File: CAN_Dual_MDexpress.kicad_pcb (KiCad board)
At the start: 2 copper layers, 105 x 100 mm, 134 parts, among them IC1 SI8650AB-B-IS1, IC2 A3921KLPTR-T, IC3 SI8650AB-B-IS1, IC4 A3921KLPTR-T, J1 Conn_01x02, J2 Conn_01x03, J3 Conn_01x05, J4 Conn_01x02, J5 Bus_mechaken_PCIexpress_x16_1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, Q1 NVMFD5C446NT1G, Q2 NVMFD5C446NT1G, Q3 NVMFD5C446NT1G, Q4 NVMFD5C446NT1G, U1 LDL1117S33TR_SOT223-4, U2 STM32F042K6Tx, U3 MCP2562-E-SN, U4 LDL1117S33TR_SOT223-4

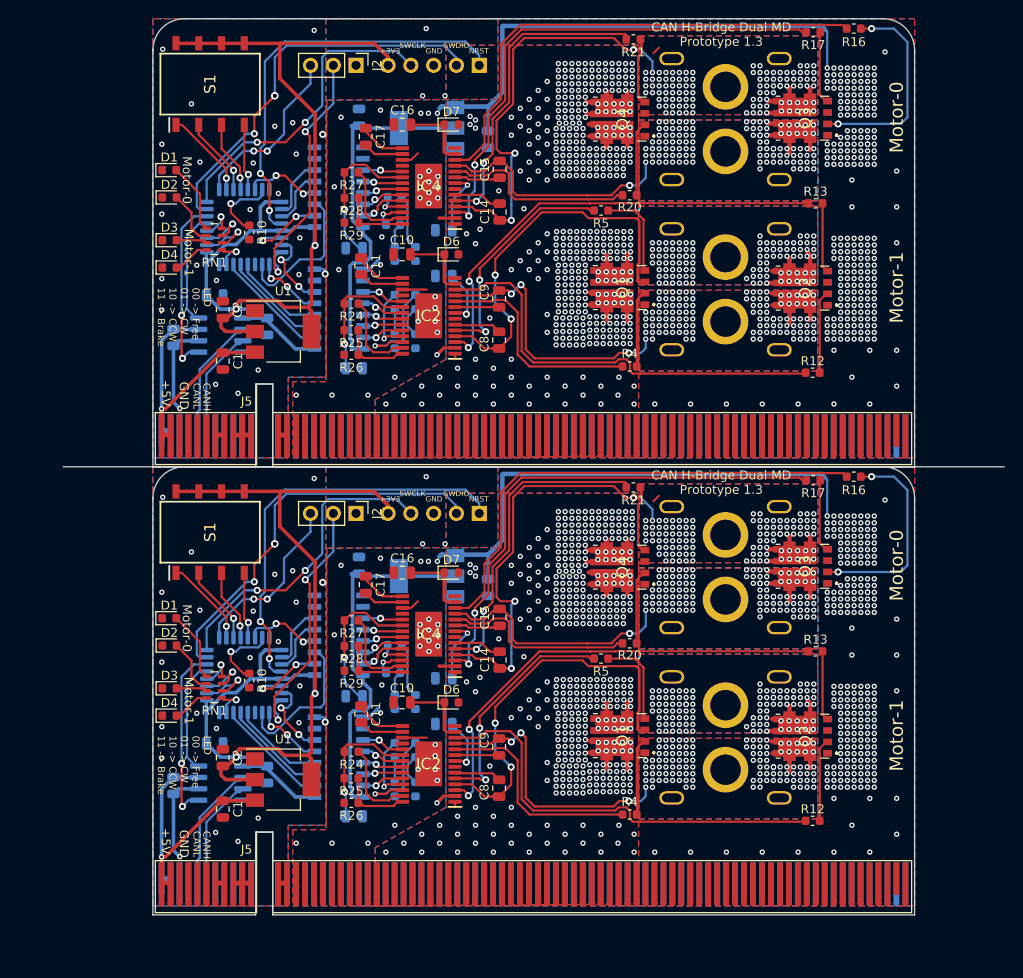
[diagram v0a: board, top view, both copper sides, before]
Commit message: Prototype 1.3
FusionPCB(12/12)
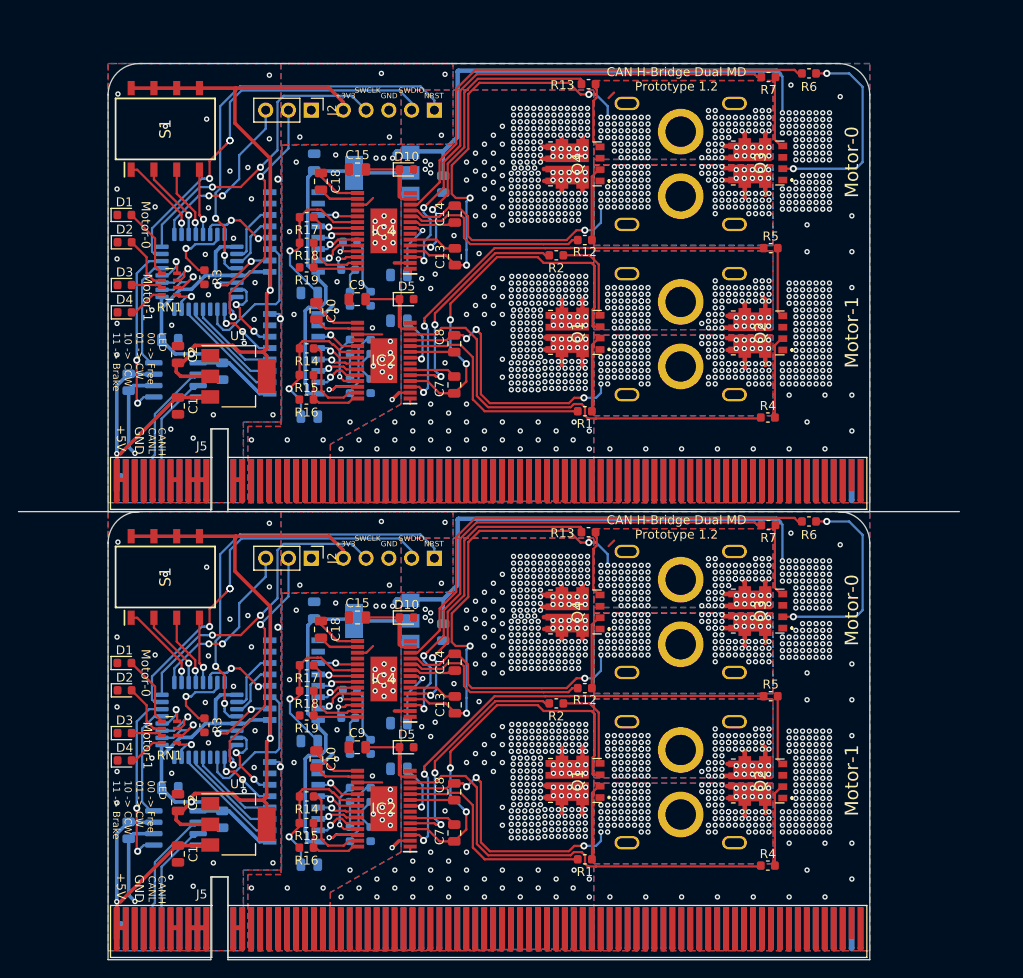
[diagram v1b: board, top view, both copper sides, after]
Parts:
- removed D11: LED, LED_SMD:LED_0603_1608Metric
- removed R20, R21: 21, Resistor_SMD:R_0603_1608Metric
- removed R24, R27: 3K, Resistor_SMD:R_0603_1608Metric
- removed R25, R28: 3.74k, Resistor_SMD:R_0603_1608Metric
- removed R26, R29: 1.2k, Resistor_SMD:R_0603_1608Metric
- removed R30, R31, R32, R33: 10K, Resistor_SMD:R_0603_1608Metric
- added D5: D, Diode_SMD:D_0603_1608Metric, F.Cu at (148.3, 66.3)
- added R1: 21, Resistor_SMD:R_0603_1608Metric, F.Cu at (168.2, 78.8)
- added R11: 10K, Resistor_SMD:R_0603_1608Metric, B.Cu at (141.8, 63.0)
- added R14: 3K, Resistor_SMD:R_0603_1608Metric, F.Cu at (137.2, 71.8)
- added R15: 3.74k, Resistor_SMD:R_0603_1608Metric, F.Cu at (137.1, 74.8)
- added R18: 3.74k, Resistor_SMD:R_0603_1608Metric, F.Cu at (137.2, 60.0)
- added R19: 1.2k, Resistor_SMD:R_0603_1608Metric, F.Cu at (137.2, 62.8)
- added R2: 21, Resistor_SMD:R_0603_1608Metric, F.Cu at (165.0, 61.4)
- added R3: 10K, Resistor_SMD:R_0603_1608Metric, F.Cu at (125.8, 63.9)
- added R6: 21, Resistor_SMD:R_0603_1608Metric, F.Cu at (193.2, 41.1)
- added R7: 21, Resistor_SMD:R_0603_1608Metric, F.Cu at (188.7, 41.5)
- added R8: 10K, Resistor_SMD:R_0603_1608Metric, B.Cu at (142.0, 71.6)
- added R9: 10K, Resistor_SMD:R_0603_1608Metric, B.Cu at (144.3, 71.6)
- C10: value 0.1uF -> 0.47uF
- C11: value 0.47uF -> 0.1uF; moved to B.Cu
- C12, C6: value 0.1uF -> 4.7uF
- C13, C7: value 4.7uF -> 0.1uF; moved to F.Cu
- C16: value 0.1uF -> 1uF; moved to B.Cu
- C17: value 0.47uF -> 4.7uF; moved to B.Cu
- C18: value 0.1uF -> 0.47uF; moved to F.Cu
- C19: value 4.7uF -> 0.1uF
- C3: value 1uF -> 0.1uF
- D10: value LED -> D; footprint LED_SMD:LED_0603_1608Metric -> Diode_SMD:D_0603_1608Metric; moved to F.Cu
- D6, D7: value D -> LED; footprint Diode_SMD:D_0603_1608Metric -> LED_SMD:LED_0603_1608Metric; moved to B.Cu
- R10: moved to B.Cu
- R16: value 21 -> 1.2k
- R17: value 21 -> 3K
- moved R16 73.8 mm to (137.1, 77.5), turned to 180 degrees
- moved R17 60.2 mm to (137.2, 57.1)
- moved C3 42.0 mm to (121.9, 70.9), turned to 180 degrees
- moved D7 30.5 mm to (144.3, 76.0), turned to 90 degrees
- moved R12 29.4 mm to (168.2, 59.7)
- moved R13 28.6 mm to (168.6, 42.3)
- moved C6 25.2 mm to (147.5, 68.7), turned to 180 degrees
- moved C19 20.4 mm to (137.5, 65.6), turned to 180 degrees
- moved R5 19.4 mm to (188.9, 60.6)
- moved D10 19.2 mm to (148.3, 51.8), turned to 0 degrees
- moved D6 18.5 mm to (142.0, 76.0), turned to 90 degrees
- moved C11 17.8 mm to (137.5, 79.4), turned to 0 degrees
- moved C5 16.6 mm to (117.3, 75.6)
- moved R4 16.4 mm to (188.6, 79.5)
- moved C15 15.9 mm to (142.8, 51.8), turned to 180 degrees
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- renumbered C11 to C10, C12 to C11, C13 to C12, C14 to C13, C15 to C14, C16 to C15, C3 to C16, C19 to C17, C17 to C18, C18 to C19, C4 to C3, C5 to C4, C6 to C5, C7 to C6, C8 to C7, C9 to C8, C10 to C9, D7 to D10, D6 to D5, D10 to D6, D11 to D7, R4 to R1, R30 to R10, R31 to R11, R20 to R12, R21 to R13, R24 to R14, R25 to R15, R26 to R16, R27 to R17, R28 to R18, R29 to R19, R5 to R2, R10 to R3, R12 to R4, R13 to R5, R16 to R6, R17 to R7, R32 to R8, R33 to R9
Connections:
- C10 pad 2: GNDPWR -> Net-(C10-Pad2)
- C10 pad 1: Net-(C11-Pad1) -> Net-(C10-Pad1)
- C10 pad 2: Net-(C11-Pad2) -> Net-(C10-Pad2)
- C11 pad 2: Net-(C11-Pad2) -> GNDPWR
- C11 pad 1: Net-(C12-Pad1) -> Net-(C11-Pad1)
- C12 pad 1: Net-(C12-Pad1) -> VREG_0
- C13 pad 1: VREG_0 -> SB_0
- C13 pad 2: GNDPWR -> Net-(C13-Pad2)
- C13 pad 2: Net-(C14-Pad2) -> Net-(C13-Pad2)
- C14 pad 1: SB_0 -> Net-(C14-Pad1)
- C14 pad 2: Net-(C14-Pad2) -> SA_0
- C14 pad 1: Net-(C15-Pad1) -> Net-(C14-Pad1)
- C15 pad 2: SA_0 -> GNDPWR
- C15 pad 1: Net-(C16-Pad1) -> Net-(C15-Pad1)
- C16 pad 1: Net-(C16-Pad1) -> VCC
- C17 pad 1: Net-(C17-Pad1) -> GNDPWR
- C17 pad 2: Net-(C17-Pad2) -> MD_3V3
- C18 pad 2: GNDPWR -> Net-(C18-Pad2)
- C18 pad 1: Net-(C17-Pad1) -> Net-(C18-Pad1)
- C18 pad 2: Net-(C17-Pad2) -> Net-(C18-Pad2)
- C19 pad 1: GNDPWR -> Net-(C19-Pad1)
- C19 pad 2: MD_3V3 -> GNDPWR
- C19 pad 1: Net-(C18-Pad1) -> Net-(C19-Pad1)
- C3 pad 1: VCC -> GND
- C3 pad 2: GNDPWR -> +3V3
- C5 pad 2: +3V3 -> +5V
- C6 pad 1: GND -> VREG_1
- C6 pad 2: +5V -> GNDPWR
- C7 pad 1: VREG_1 -> SB_1
- C7 pad 2: GNDPWR -> Net-(C7-Pad2)
- C7 pad 2: Net-(C8-Pad2) -> Net-(C7-Pad2)
- C8 pad 1: SB_1 -> SA_1
- C8 pad 2: Net-(C9-Pad2) -> Net-(C8-Pad2)
- C9 pad 1: SA_1 -> Net-(C9-Pad1)
- C9 pad 2: Net-(C9-Pad2) -> GNDPWR
- C9 pad 1: Net-(C10-Pad1) -> Net-(C9-Pad1)
- D10 pad 1: GNDPWR -> Net-(C15-Pad1)
- D10 pad 2: Net-(D10-Pad2) -> VCC
- D10 pad 1: Net-(C16-Pad1) -> Net-(C15-Pad1)
- D5 pad 1: Net-(C10-Pad1) -> Net-(C9-Pad1)
- D6 pad 1: Net-(C10-Pad1) -> GNDPWR
- D6 pad 2: VCC -> Net-(D6-Pad2)
- D6 pad 2: Net-(D10-Pad2) -> Net-(D6-Pad2)
- D7 pad 1: Net-(C16-Pad1) -> GNDPWR
- D7 pad 2: VCC -> Net-(D7-Pad2)
- D7 pad 2: Net-(D11-Pad2) -> Net-(D7-Pad2)
- IC2 pad 13: Net-(C10-Pad1) -> Net-(C9-Pad1) (x2)
- IC2 pad 15: Net-(C11-Pad1) -> Net-(C10-Pad1) (x2)
- IC2 pad 16: Net-(C11-Pad2) -> Net-(C10-Pad2) (x2)
- IC2 pad 20: Net-(C12-Pad1) -> Net-(C11-Pad1) (x2)
- IC2 pad 6: Net-(C8-Pad2) -> Net-(C7-Pad2) (x2)
- IC2 pad 9: Net-(C9-Pad2) -> Net-(C8-Pad2) (x2)
- IC4 pad 13: Net-(C16-Pad1) -> Net-(C15-Pad1) (x2)
- IC4 pad 15: Net-(C17-Pad1) -> Net-(C18-Pad1) (x2)
- IC4 pad 16: Net-(C17-Pad2) -> Net-(C18-Pad2) (x2)
- IC4 pad 20: Net-(C18-Pad1) -> Net-(C19-Pad1) (x2)
- IC4 pad 6: Net-(C14-Pad2) -> Net-(C13-Pad2) (x2)
- IC4 pad 9: Net-(C15-Pad1) -> Net-(C14-Pad1) (x2)
- R10 pad 1: /BOOT -> MD_FF1_0
- R10 pad 2: GND -> Net-(D8-Pad2)
- R12 pad 1: GLA_1 -> GHA_0
- R12 pad 2: Net-(Q2-Pad2) -> Net-(Q4-Pad2)
- R13 pad 1: Net-(Q2-Pad4) -> Net-(Q4-Pad4)
- R13 pad 2: GLB_1 -> GHB_0
- R14 pad 2: Net-(C12-Pad1) -> Net-(C11-Pad1)
- R15 pad 2: Net-(C12-Pad1) -> Net-(C11-Pad1)
- R16 pad 1: GLA_0 -> Net-(IC2-Pad28)
- R16 pad 2: Net-(Q3-Pad2) -> GNDPWR
- R17 pad 1: Net-(Q3-Pad4) -> Net-(IC4-Pad27)
- R17 pad 2: GLB_0 -> Net-(C19-Pad1)
- R17 pad 2: Net-(C18-Pad1) -> Net-(C19-Pad1)
- R18 pad 2: Net-(C18-Pad1) -> Net-(C19-Pad1)
- R4 pad 1: GHA_1 -> GLA_1
- R4 pad 2: Net-(Q1-Pad2) -> Net-(Q2-Pad2)
- R5 pad 1: Net-(Q1-Pad4) -> Net-(Q2-Pad4)
- R5 pad 2: GHB_1 -> GLB_1
- R8 pad 2: Net-(D10-Pad2) -> Net-(D6-Pad2)
- R9 pad 2: Net-(D11-Pad2) -> Net-(D7-Pad2)
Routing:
- net Net-(C19-Pad1): track 0.00 -> 36.0 mm, vias 0 -> 2
- net Net-(C12-Pad1): track 29.2 -> 0.00 mm, vias 2 -> 0
- net Net-(C18-Pad1): track 33.8 -> 11.0 mm, vias 2 -> 0
- net Net-(C9-Pad1): track 0.00 -> 22.3 mm
- net Net-(C16-Pad1): track 22.3 -> 0.00 mm
- net Net-(C11-Pad1): track 11.4 -> 32.8 mm, vias 0 -> 2
- net Net-(C17-Pad2): track 15.2 -> 0.00 mm
- net Net-(C18-Pad2): track 0.00 -> 15.2 mm
- net Net-(C15-Pad1): track 9.33 -> 22.3 mm
- net Net-(C17-Pad1): track 11.0 -> 0.00 mm
- net Net-(C10-Pad1): track 22.3 -> 11.4 mm
- net Net-(C14-Pad2): track 10.8 -> 0.00 mm
- net Net-(C13-Pad2): track 0.00 -> 10.8 mm
- net Net-(C7-Pad2): track 0.00 -> 10.5 mm
- net Net-(C10-Pad2): track 0.00 -> 10.2 mm
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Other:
- board text added: "CAN H-Bridge Dual MD Prototype 1.2"
- board text removed: "CAN H-Bridge Dual MD Prototype 1.3"

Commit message: clean
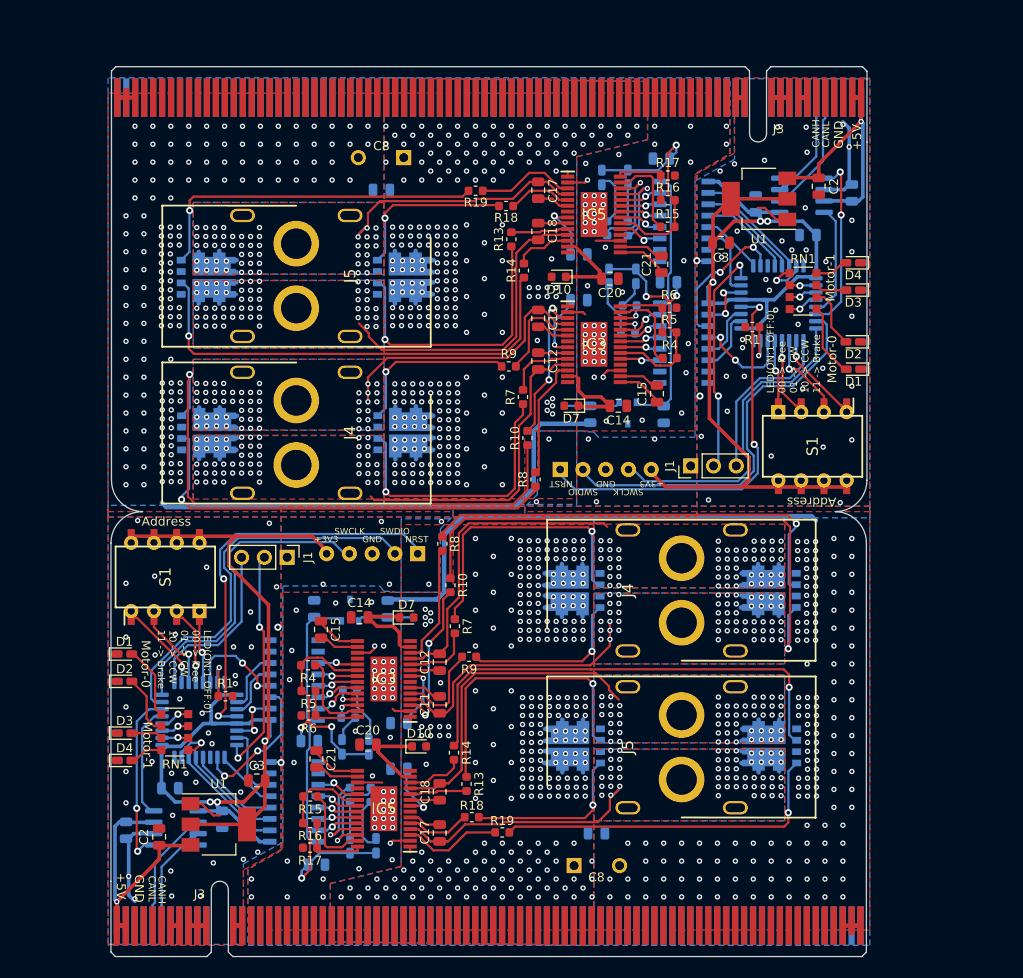
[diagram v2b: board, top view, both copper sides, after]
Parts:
- removed the C8 at (153.6, 71.3)
- removed the C9 at (142.8, 66.3)
- removed the IC2 at (145.8, 73.2)
- removed the J1 at (178.9, 70.2)
- removed the J2 at (137.7, 45.2)
- removed the J2 at (137.7, 95.2)
- removed the J3 at (151.4, 45.2)
- removed the J3 at (151.4, 95.2)
- removed U4 (x2): LDL1117S33TR_SOT223-4, Package_TO_SOT_SMD:SOT-223-3_TabPin2
- added C20: 0.1u, Capacitor_SMD:C_0805_2012Metric, F.Cu at (171.0, 64.0)
- added C21: 0.47u, Capacitor_SMD:C_0805_2012Metric, F.Cu at (176.8, 62.4)
- added C8: 1000u, Connector_PinSocket_2.54mm:PinSocket_1x02_P2.54mm_Vertical, B.Cu at (148.0, 50.5)
- added C8: 1000u, Connector_PinSocket_2.54mm:PinSocket_1x02_P2.54mm_Vertical, B.Cu at (167.0, 129.5)
- added C9: 10u, Capacitor_SMD:C_0805_2012Metric, B.Cu at (145.5, 54.1)
- added C9: 10u, Capacitor_SMD:C_0805_2012Metric, B.Cu at (169.5, 125.9)
- added IC2: AP7381-50SA-7, SamacSys_Parts:SOT96P240X105-3N, B.Cu at (173.0, 79.0)
- added IC2: AP7381-50SA-7, SamacSys_Parts:SOT96P240X105-3N, B.Cu at (142.0, 101.0)
- added IC5: A3921KLPTR-T, SamacSys_Parts:SOP65P640X120-29N, F.Cu at (169.2, 56.8)
- added J1: Conn_01x03, Connector_PinHeader_2.54mm:PinHeader_1x03_P2.54mm_Vertical, F.Cu at (180.0, 84.9)
- added J1: Conn_01x03, Connector_PinHeader_2.54mm:PinHeader_1x03_P2.54mm_Vertical, F.Cu at (135.0, 95.1)
- added J2: Conn_01x05, Connector_PinHeader_2.54mm:PinHeader_1x05_P2.54mm_Vertical, B.Cu at (165.4, 85.3)
- added J2: Conn_01x05, Connector_PinHeader_2.54mm:PinHeader_1x05_P2.54mm_Vertical, B.Cu at (149.6, 94.7)
- added J3: Bus_mechaken_PCIexpress_x16_164_Position, PCIe:BUS_mechaken_PCIexpress_x16, F.Cu at (199.0, 43.8)
- added S2: DIPSW, Package_DIP:DIP-8_W7.62mm, B.Cu at (189.8, 78.9)
- added S2: DIPSW, Package_DIP:DIP-8_W7.62mm, B.Cu at (125.2, 101.1)
- C1: value 1uF -> 0.1u; moved to B.Cu
- C1: renamed from C3; value 0.1uF -> 0.1u
- C10: value 0.47uF -> 4.7u; moved to B.Cu
- C10: renamed from C12; value 4.7uF -> 4.7u
- C11, C3: value 0.1uF -> 4.7u; moved to F.Cu
- C11: renamed from C13; value 0.1uF -> 4.7u
- C12, C17: value 4.7uF -> 4.7u; moved to F.Cu
- C12: renamed from C14; value 0.1uF -> 4.7u
- C13, C7: value 0.1uF -> 0.1u; moved to B.Cu
- C13: renamed from C19; value 0.1uF -> 0.1u
- C14, C19, C4: value 0.1uF -> 0.1u
- C14: renamed from C15; value 0.1uF -> 0.1u
- C15: value 0.1uF -> 0.47u
- C15: renamed from C18; value 0.47uF -> 0.47u
- C16: value 1uF -> 4.7u
- C16: renamed from C6; value 4.7uF -> 4.7u
- C17: renamed from C7; value 0.1uF -> 4.7u
- C18: value 0.47uF -> 4.7u
- C18: renamed from C8; value 0.1uF -> 4.7u
- C19: renamed from C11; value 0.1uF -> 0.1u
- C2: value 4.7uF -> 1u
- C2: renamed from C1; value 1uF -> 1u
- C20: renamed from C9; value 0.1uF -> 0.1u
- C21: renamed from C10; value 0.47uF -> 0.47u
- C3: renamed from C2; value 4.7uF -> 4.7u
- C4: renamed from C5; value 0.1uF -> 0.1u
- C5: value 0.1uF -> 1u
- C5: renamed from C16; value 1uF -> 1u
- C6: value 4.7uF -> 2.2u
- C6: renamed from C17; value 4.7uF -> 2.2u
- C7: renamed from C4; value 0.1uF -> 0.1u
- D1 (x2), D2 (x2), D3 (x2), D4 (x2), D6, D8, D9: footprint LED_SMD:LED_0603_1608Metric -> LED_SMD:LED_0603_1608Metric_Castellated
- D5: value D -> LED; footprint Diode_SMD:D_0603_1608Metric -> LED_SMD:LED_0603_1608Metric_Castellated; moved to B.Cu
- D5: renamed from D8; footprint LED_SMD:LED_0603_1608Metric -> LED_SMD:LED_0603_1608Metric_Castellated
- D6: renamed from D9; footprint LED_SMD:LED_0603_1608Metric -> LED_SMD:LED_0603_1608Metric_Castellated
- D7: value LED -> D; footprint LED_SMD:LED_0603_1608Metric -> Diode_SMD:D_0603_1608Metric; moved to F.Cu
- D8: renamed from D6; footprint LED_SMD:LED_0603_1608Metric -> LED_SMD:LED_0603_1608Metric_Castellated
- D9: renamed from D7; footprint LED_SMD:LED_0603_1608Metric -> LED_SMD:LED_0603_1608Metric_Castellated
- IC3: value SI8650AB-B-IS1 -> A3921KLPTR-T; footprint SamacSys_Parts:SOIC127P600X175-16N -> SamacSys_Parts:SOP65P640X120-29N; moved to F.Cu
- IC4: value A3921KLPTR-T -> SI8650AB-B-IS1; footprint SamacSys_Parts:SOP65P640X120-29N -> SamacSys_Parts:SOIC127P600X175-16N; moved to B.Cu
- J3: renamed from J5; footprint PCIe:BUS_mechaken_PCIexpress_x16_164_Position -> PCIe:BUS_mechaken_PCIexpress_x16
- J4 (x2): moved to F.Cu
- J5: value Bus_mechaken_PCIexpress_x16_164_Position -> Conn_01x02; footprint PCIe:BUS_mechaken_PCIexpress_x16_164_Position -> XT60:XT60PW_Reversible
- J5: renamed from J1; moved to F.Cu
- Q1, Q2, Q3, Q4: moved to B.Cu
- Q1: renamed from Q4; moved to B.Cu
- Q2: renamed from Q3; moved to B.Cu
- Q3: renamed from Q1; moved to B.Cu
- Q4: renamed from Q2; moved to B.Cu
- R1, R5: value 21 -> 10k
- R1: renamed from R3; value 10K -> 10k
- R10, R8, R9: value 10K -> 21; moved to F.Cu
- R11: value 10K -> 2.2k
- R11: renamed from R8; value 10K -> 2.2k
- R12, R2: value 21 -> 2.2k; moved to B.Cu
- R12: renamed from R9; value 10K -> 2.2k
- R14: value 3K -> 21
- R15: value 3.74k -> 3k
- R15: renamed from R14; value 3K -> 3k
- R16: value 1.2k -> 10k
- R16: renamed from R15; value 3.74k -> 10k
- R17: value 3K -> 2.2k
- R17: renamed from R16; value 1.2k -> 2.2k
- R18: value 3.74k -> 21
- R19: value 1.2k -> 21
- R2: renamed from R10; value 10K -> 2.2k
- R3: value 10K -> 2.2k; moved to B.Cu
- R3: renamed from R11; value 10K -> 2.2k
- R4: value 21 -> 3k
- R4: renamed from R17; value 3K -> 3k
- R5: renamed from R18; value 3.74k -> 10k
- R6: value 21 -> 2.2k
- R6: renamed from R19; value 1.2k -> 2.2k
- RN1 (x2): value R_Pack04 -> 2.2k; footprint Resistor_SMD:R_Array_Concave_4x0603 -> Resistor_SMD:R_Array_Convex_4x1206
- U1 (x2): value LDL1117S33TR_SOT223-4 -> LDL1117S33R_SOT223-4
- moved D1 83.2 mm to (198.2, 74.1), turned to 180 degrees
- moved D2 82.1 mm to (198.2, 71.1), turned to 180 degrees
- moved D4 81.5 mm to (198.2, 62.2), turned to 180 degrees
- moved D3 81.3 mm to (198.2, 65.3), turned to 180 degrees
- moved S1 80.4 mm to (193.6, 82.7), turned to 270 degrees
- moved C2 73.9 mm to (194.3, 53.7)
- moved C4 73.0 mm to (198.0, 54.4), turned to 270 degrees
- moved C1 72.8 mm to (193.1, 59.1), turned to 0 degrees
- moved U3 72.8 mm to (192.4, 54.7), turned to 180 degrees
- moved RN1 70.7 mm to (192.6, 65.4), turned to 180 degrees
- moved U2 64.7 mm to (189.8, 66.8), turned to 0 degrees
- moved Q2 63.1 mm to (125.7, 81.2)
- moved C3 62.5 mm to (183.4, 60.0)
- moved U1 61.4 mm to (187.7, 55.1), turned to 180 degrees
- moved J4 52.3 mm to (136.0, 81.2)
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- renumbered D5 to D10, D10 to D7, IC3 to IC1, IC4 to IC3, IC1 to IC4, IC2 to IC5, R7 to R10, R2 to R13, R5 to R14, R1 to R18, R4 to R19, R13 to R7, R6 to R8, R12 to R9
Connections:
- C1 pad 1: +5V -> GND
- C1 pad 2: GND -> +3V3
- C10 pad 1: Net-(C10-Pad1) -> VREG_0
- C10 pad 2: Net-(C10-Pad2) -> GNDPWR
- C11 pad 1: Net-(C11-Pad1) -> SB_0
- C11 pad 2: GNDPWR -> Net-(C11-Pad2)
- C11 pad 2: Net-(C13-Pad2) -> Net-(C11-Pad2)
- C12 pad 1: VREG_0 -> Net-(C12-Pad1)
- C12 pad 2: GNDPWR -> SA_0
- C12 pad 1: Net-(C14-Pad1) -> Net-(C12-Pad1)
- C13 pad 1: SB_0 -> V5_0
- C13 pad 2: Net-(C13-Pad2) -> GNDPWR
- C13 pad 1: Net-(C19-Pad1) -> V5_0
- C14 pad 2: SA_0 -> GNDPWR
- C14 pad 1: Net-(C15-Pad1) -> Net-(C14-Pad1)
- C15 pad 2: GNDPWR -> Net-(C15-Pad2)
- C15 pad 1: Net-(C18-Pad1) -> Net-(C15-Pad1)
- C15 pad 2: Net-(C18-Pad2) -> Net-(C15-Pad2)
- C16 pad 1: VCC -> VREG_1
- C17 pad 1: GNDPWR -> SB_1
- C17 pad 2: MD_3V3 -> Net-(C17-Pad2)
- C17 pad 2: Net-(C7-Pad2) -> Net-(C17-Pad2)
- C18 pad 1: Net-(C18-Pad1) -> SA_1
- C18 pad 2: Net-(C8-Pad2) -> Net-(C18-Pad2)
- C19 pad 1: Net-(C19-Pad1) -> V5_1
- C19 pad 1: Net-(C11-Pad1) -> V5_1
- C2 pad 1: GND -> +5V
- C2 pad 2: +3V3 -> GND
- C20 pad 1: Net-(C9-Pad1) -> Net-(C20-Pad1)
- C21 pad 1: Net-(C10-Pad1) -> Net-(C21-Pad1)
- C21 pad 2: Net-(C10-Pad2) -> Net-(C21-Pad2)
- C4 pad 2: +3V3 -> +5V
- C5 pad 1: GND -> VCC
- C5 pad 2: +5V -> GNDPWR
- C6 pad 1: VREG_1 -> GNDPWR
- C6 pad 2: GNDPWR -> MD_3V3
- C7 pad 1: SB_1 -> GND
- C7 pad 2: Net-(C7-Pad2) -> +3V3
- D10 pad 1: Net-(C15-Pad1) -> Net-(C20-Pad1)
- D10 pad 1: Net-(C9-Pad1) -> Net-(C20-Pad1)
- D5 pad 1: Net-(C9-Pad1) -> Net-(D5-Pad1)
- D5 pad 2: VCC -> V5_0
- D5 pad 1: GNDPWR -> Net-(D5-Pad1)
- D5 pad 2: Net-(D8-Pad2) -> V5_0
- D6 pad 1: GNDPWR -> Net-(D6-Pad1) (x2)
- D6 pad 2: Net-(D6-Pad2) -> V5_0
- D6 pad 2: Net-(D9-Pad2) -> V5_0
- D7 pad 1: GNDPWR -> Net-(C14-Pad1)
- D7 pad 2: Net-(D7-Pad2) -> VCC
- D7 pad 1: Net-(C15-Pad1) -> Net-(C14-Pad1)
- D8 pad 1: GNDPWR -> Net-(D8-Pad1) (x2)
- D8 pad 2: Net-(D8-Pad2) -> V5_1
- D8 pad 2: Net-(D6-Pad2) -> V5_1
- D9 pad 1: GNDPWR -> Net-(D9-Pad1) (x2)
- D9 pad 2: Net-(D9-Pad2) -> V5_1
- D9 pad 2: Net-(D7-Pad2) -> V5_1
- IC1 pad 10: (no net) -> Net-(IC1-Pad10) (x2)
- IC1 pad 11: MD_PHASE_1 -> MD_PHASE_0
- IC1 pad 12: MD_SR_1 -> MD_SR_0
- IC1 pad 13: MD_PWML_1 -> MD_PWML_0
- IC1 pad 14: MD_PWMH_1 -> MD_PWMH_0
- IC1 pad 15: MD_RESET_1 -> MD_RESET_0
- IC1 pad 2: IC_RESET_1 -> IC_RESET_0
- IC1 pad 3: IC_PWMH_1 -> IC_PWMH_0
- IC1 pad 4: IC_PWML_1 -> IC_PWML_0
- IC1 pad 5: IC_SR_1 -> IC_SR_0
- IC1 pad 6: IC_PHASE_1 -> IC_PHASE_0
- IC1 pad 7: (no net) -> Net-(IC1-Pad7) (x2)
- IC3 pad 1: +3V3 -> VCC
- IC3 pad 10: (no net) -> GHA_0
- IC3 pad 11: MD_PHASE_0 -> SA_0
- IC3 pad 12: MD_SR_0 -> GLA_0
- IC3 pad 13: MD_PWML_0 -> Net-(C14-Pad1)
- IC3 pad 14: MD_PWMH_0 -> Net-(IC3-Pad14)
- IC3 pad 15: MD_RESET_0 -> Net-(C15-Pad1)
- IC3 pad 16: MD_3V3 -> Net-(C15-Pad2)
- IC3 pad 2: IC_RESET_0 -> GNDPWR
- IC3 pad 3: IC_PWMH_0 -> GLB_0
- IC3 pad 4: IC_PWML_0 -> SB_0
- IC3 pad 5: IC_SR_0 -> GHB_0
- IC3 pad 6: IC_PHASE_0 -> Net-(C11-Pad2)
- IC3 pad 7: (no net) -> Net-(IC3-Pad7) (x2)
- IC3 pad 8: GND -> VREG_0
- IC3 pad 9: GNDPWR -> Net-(C12-Pad1)
- IC3 pad 13: Net-(C15-Pad1) -> Net-(C14-Pad1)
- IC3 pad 14: (no net) -> Net-(IC3-Pad14)
- IC3 pad 15: Net-(C18-Pad1) -> Net-(C15-Pad1)
- IC3 pad 16: Net-(C18-Pad2) -> Net-(C15-Pad2)
- IC3 pad 18: (no net) -> Net-(IC3-Pad18)
- IC3 pad 20: Net-(C19-Pad1) -> V5_0
- IC3 pad 27: Net-(IC4-Pad27) -> Net-(IC3-Pad27)
- IC3 pad 28: Net-(IC4-Pad28) -> Net-(IC3-Pad28)
- IC3 pad 6: Net-(C13-Pad2) -> Net-(C11-Pad2)
- IC3 pad 9: Net-(C14-Pad1) -> Net-(C12-Pad1)
- IC4 pad 1: VCC -> +3V3
- IC4 pad 10: GHA_0 -> Net-(IC4-Pad10)
- IC4 pad 11: SA_0 -> MD_PHASE_1
- IC4 pad 12: GLA_0 -> MD_SR_1
- IC4 pad 13: Net-(C15-Pad1) -> MD_PWML_1
- IC4 pad 14: (no net) -> MD_PWMH_1
- IC4 pad 15: Net-(C18-Pad1) -> MD_RESET_1
- IC4 pad 16: Net-(C18-Pad2) -> MD_3V3
- IC4 pad 2: GNDPWR -> IC_RESET_1
- IC4 pad 3: GLB_0 -> IC_PWMH_1
- IC4 pad 4: SB_0 -> IC_PWML_1
- IC4 pad 5: GHB_0 -> IC_SR_1
- IC4 pad 6: Net-(C13-Pad2) -> IC_PHASE_1
- IC4 pad 7: (no net) -> Net-(IC4-Pad7) (x2)
- IC4 pad 8: VREG_0 -> GND
- IC4 pad 9: Net-(C14-Pad1) -> GNDPWR
- IC4 pad 10: (no net) -> Net-(IC4-Pad10)
- IC5 pad 13: Net-(C9-Pad1) -> Net-(C20-Pad1)
- IC5 pad 14: (no net) -> Net-(IC5-Pad14)
- IC5 pad 15: Net-(C10-Pad1) -> Net-(C21-Pad1)
- IC5 pad 16: Net-(C10-Pad2) -> Net-(C21-Pad2)
- IC5 pad 18: (no net) -> Net-(IC5-Pad18)
- IC5 pad 20: Net-(C11-Pad1) -> V5_1
- IC5 pad 27: Net-(IC2-Pad27) -> Net-(IC5-Pad27)
- IC5 pad 28: Net-(IC2-Pad28) -> Net-(IC5-Pad28)
- IC5 pad 6: Net-(C7-Pad2) -> Net-(C17-Pad2)
- IC5 pad 7: (no net) -> Net-(IC5-Pad7)
- IC5 pad 9: Net-(C8-Pad2) -> Net-(C18-Pad2)
- J3 pad A5: Net-(J5-PadA5) -> Net-(J3-PadA5)
- J3 pad A6: Net-(J5-PadA6) -> Net-(J3-PadA6)
- J3 pad A7: Net-(J5-PadA7) -> Net-(J3-PadA7)
- J3 pad B3: Net-(J5-PadB3) -> Net-(J3-PadB3)
- J3 pad B4: Net-(J5-PadB4) -> Net-(J3-PadB4)
- J3 pad B5: Net-(J5-PadB5) -> Net-(J3-PadB5)
- J3 pad B6: Net-(J5-PadB6) -> Net-(J3-PadB6)
- J3 pad B7: Net-(J5-PadB7) -> Net-(J3-PadB7)
- Q1 pad 1: SA_1 -> SA_0
- Q1 pad 3: SB_1 -> SB_0
- Q1 pad 2: Net-(Q4-Pad2) -> Net-(Q1-Pad2)
- Q1 pad 4: Net-(Q4-Pad4) -> Net-(Q1-Pad4)
- Q2 pad 5: SB_1 -> SB_0
- Q2 pad 6: SA_1 -> SA_0
- Q2 pad 2: Net-(Q3-Pad2) -> Net-(Q2-Pad2)
- Q2 pad 4: Net-(Q3-Pad4) -> Net-(Q2-Pad4)
- Q3 pad 1: GNDPWR -> SA_1
- Q3 pad 3: GNDPWR -> SB_1
- Q3 pad 5: SB_0 -> VCC
- Q3 pad 6: SA_0 -> VCC
- Q3 pad 2: Net-(Q1-Pad2) -> Net-(Q3-Pad2)
- Q3 pad 4: Net-(Q1-Pad4) -> Net-(Q3-Pad4)
- Q4 pad 1: SA_0 -> GNDPWR
- Q4 pad 3: SB_0 -> GNDPWR
- Q4 pad 5: VCC -> SB_1
- Q4 pad 6: VCC -> SA_1
- Q4 pad 2: Net-(Q2-Pad2) -> Net-(Q4-Pad2)
- Q4 pad 4: Net-(Q2-Pad4) -> Net-(Q4-Pad4)
- R1 pad 1: GHA_1 -> /BOOT
- R1 pad 2: Net-(Q1-Pad2) -> GND
- R10 pad 1: MD_FF1_0 -> Net-(Q2-Pad4)
- R10 pad 2: Net-(D8-Pad2) -> GLB_0
- R10 pad 1: Net-(Q3-Pad4) -> Net-(Q2-Pad4)
- R11 pad 1: MD_FF2_0 -> MD_FF2_1
- R11 pad 2: Net-(D9-Pad2) -> Net-(D8-Pad1)
- R11 pad 2: Net-(D6-Pad2) -> Net-(D8-Pad1)
- R12 pad 1: GHA_0 -> MD_FF1_1
- R12 pad 2: Net-(Q4-Pad2) -> Net-(D9-Pad1)
- R12 pad 2: Net-(D7-Pad2) -> Net-(D9-Pad1)
- R13 pad 1: Net-(Q4-Pad4) -> Net-(Q3-Pad2)
- R13 pad 2: GHB_0 -> GHA_1
- R13 pad 1: Net-(Q1-Pad4) -> Net-(Q3-Pad2)
- R13 pad 2: GHB_1 -> GHA_1
- R14 pad 1: Net-(IC2-Pad27) -> Net-(Q4-Pad2)
- R14 pad 2: Net-(C11-Pad1) -> GLA_1
- R14 pad 1: Net-(Q2-Pad4) -> Net-(Q4-Pad2)
- R14 pad 2: GLB_1 -> GLA_1
- R15 pad 1: Net-(IC2-Pad28) -> Net-(IC5-Pad27)
- R15 pad 2: Net-(C11-Pad1) -> V5_1 (x2)
- R15 pad 1: Net-(IC2-Pad27) -> Net-(IC5-Pad27)
- R16 pad 1: Net-(IC2-Pad28) -> Net-(IC5-Pad28) (x2)
- R16 pad 2: GNDPWR -> V5_1
- R16 pad 2: Net-(C11-Pad1) -> V5_1
- R17 pad 1: Net-(IC4-Pad27) -> Net-(IC5-Pad28)
- R17 pad 2: Net-(C19-Pad1) -> GNDPWR
- R17 pad 1: Net-(IC2-Pad28) -> Net-(IC5-Pad28)
- R18 pad 1: Net-(IC4-Pad28) -> GHB_1
- R18 pad 2: Net-(C19-Pad1) -> Net-(Q3-Pad4)
- R18 pad 1: GHA_1 -> GHB_1
- R18 pad 2: Net-(Q1-Pad2) -> Net-(Q3-Pad4)
- R19 pad 1: Net-(IC4-Pad28) -> GLB_1
- R19 pad 2: GNDPWR -> Net-(Q4-Pad4)
- R19 pad 1: GLA_1 -> GLB_1
- R19 pad 2: Net-(Q2-Pad2) -> Net-(Q4-Pad4)
- R2 pad 1: Net-(Q1-Pad4) -> MD_FF1_0
- R2 pad 2: GHB_1 -> Net-(D5-Pad1)
- R2 pad 2: Net-(D8-Pad2) -> Net-(D5-Pad1)
- R3 pad 1: /BOOT -> MD_FF2_0
- R3 pad 2: GND -> Net-(D6-Pad1)
- R3 pad 2: Net-(D9-Pad2) -> Net-(D6-Pad1)
- R4 pad 1: GLA_1 -> Net-(IC3-Pad27)
- R4 pad 2: Net-(Q2-Pad2) -> V5_0
- R4 pad 1: Net-(IC4-Pad27) -> Net-(IC3-Pad27)
- R4 pad 2: Net-(C19-Pad1) -> V5_0
- R5 pad 1: Net-(Q2-Pad4) -> Net-(IC3-Pad28)
- R5 pad 2: GLB_1 -> V5_0
- R5 pad 1: Net-(IC4-Pad28) -> Net-(IC3-Pad28)
- R5 pad 2: Net-(C19-Pad1) -> V5_0
- R6 pad 1: GLA_0 -> Net-(IC3-Pad28)
- R6 pad 2: Net-(Q3-Pad2) -> GNDPWR
- R6 pad 1: Net-(IC4-Pad28) -> Net-(IC3-Pad28)
- R7 pad 1: Net-(Q3-Pad4) -> Net-(Q1-Pad2)
- R7 pad 2: GLB_0 -> GHA_0
- R7 pad 1: Net-(Q4-Pad4) -> Net-(Q1-Pad2)
- R7 pad 2: GHB_0 -> GHA_0
- R8 pad 1: MD_FF2_1 -> GLA_0
- R8 pad 2: Net-(D6-Pad2) -> Net-(Q2-Pad2)
- R8 pad 2: Net-(Q3-Pad2) -> Net-(Q2-Pad2)
- R9 pad 1: MD_FF1_1 -> GHB_0
- R9 pad 2: Net-(D7-Pad2) -> Net-(Q1-Pad4)
- R9 pad 1: GHA_0 -> GHB_0
- R9 pad 2: Net-(Q4-Pad2) -> Net-(Q1-Pad4)
- U2 pad 11: (no net) -> Net-(U2-Pad11) (x2)
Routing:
- net Net-(Q2-Pad4): track 15.7 -> 125.2 mm, vias 0 -> 2
- net Net-(Q4-Pad2): track 16.6 -> 105.2 mm, vias 0 -> 2
- net GLA_0: track 110.3 -> 26.9 mm
- net GLA_1: track 96.2 -> 13.0 mm
- net GLB_1: track 103.2 -> 22.1 mm, vias 4 -> 0
- net GLB_0: track 114.9 -> 34.3 mm
- net Net-(Q2-Pad2): track 18.5 -> 98.2 mm, vias 0 -> 2
- net Net-(Q4-Pad4): track 16.0 -> 77.2 mm, vias 0 -> 2
- net V5_1: track 0.00 -> 53.6 mm, vias 0 -> 2
- net SB_0: track 116.1 -> 62.8 mm, vias 218 -> 104
- net V5_0: track 0.00 -> 52.0 mm, vias 0 -> 4
- net GHB_0: track 71.5 -> 21.3 mm, vias 4 -> 0
- net SB_1: track 105.3 -> 59.1 mm, vias 206 -> 104
- net Net-(Q1-Pad2): track 17.0 -> 62.5 mm, vias 0 -> 2
- net GHB_1: track 53.2 -> 14.4 mm, vias 4 -> 0
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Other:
- board size 105 x 100 mm -> 84.4 x 82.5 mm
- board text added: "Address"
- board text added: "CAN Dual H-Bridge MD Prototype 1.3"
- board text added: "Conthrough"
- board text added: "LED(ON:1 OFF:0) 00 -> Free 01 -> CW 10 -> CCW 11 -> Brake"
- board text removed: "CAN H-Bridge Dual MD Prototype 1.2"
- board text removed: "LED 00 -> Free 01 -> CW 10 -> CCW 11 -> Brake"
